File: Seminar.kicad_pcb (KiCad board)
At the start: 2 copper layers, 185.7 x 157.2 mm, 40 parts, among them J1 Screw_Terminal_01x02, J1 USB_B_Mini, SW1 SW_Push, SW2 SW_Push, U1 NUCLEO64-F446RE, U2 PCF8574AP, U3 LM2574N-5, U3 TPS61023DRLR, U4 TP4056

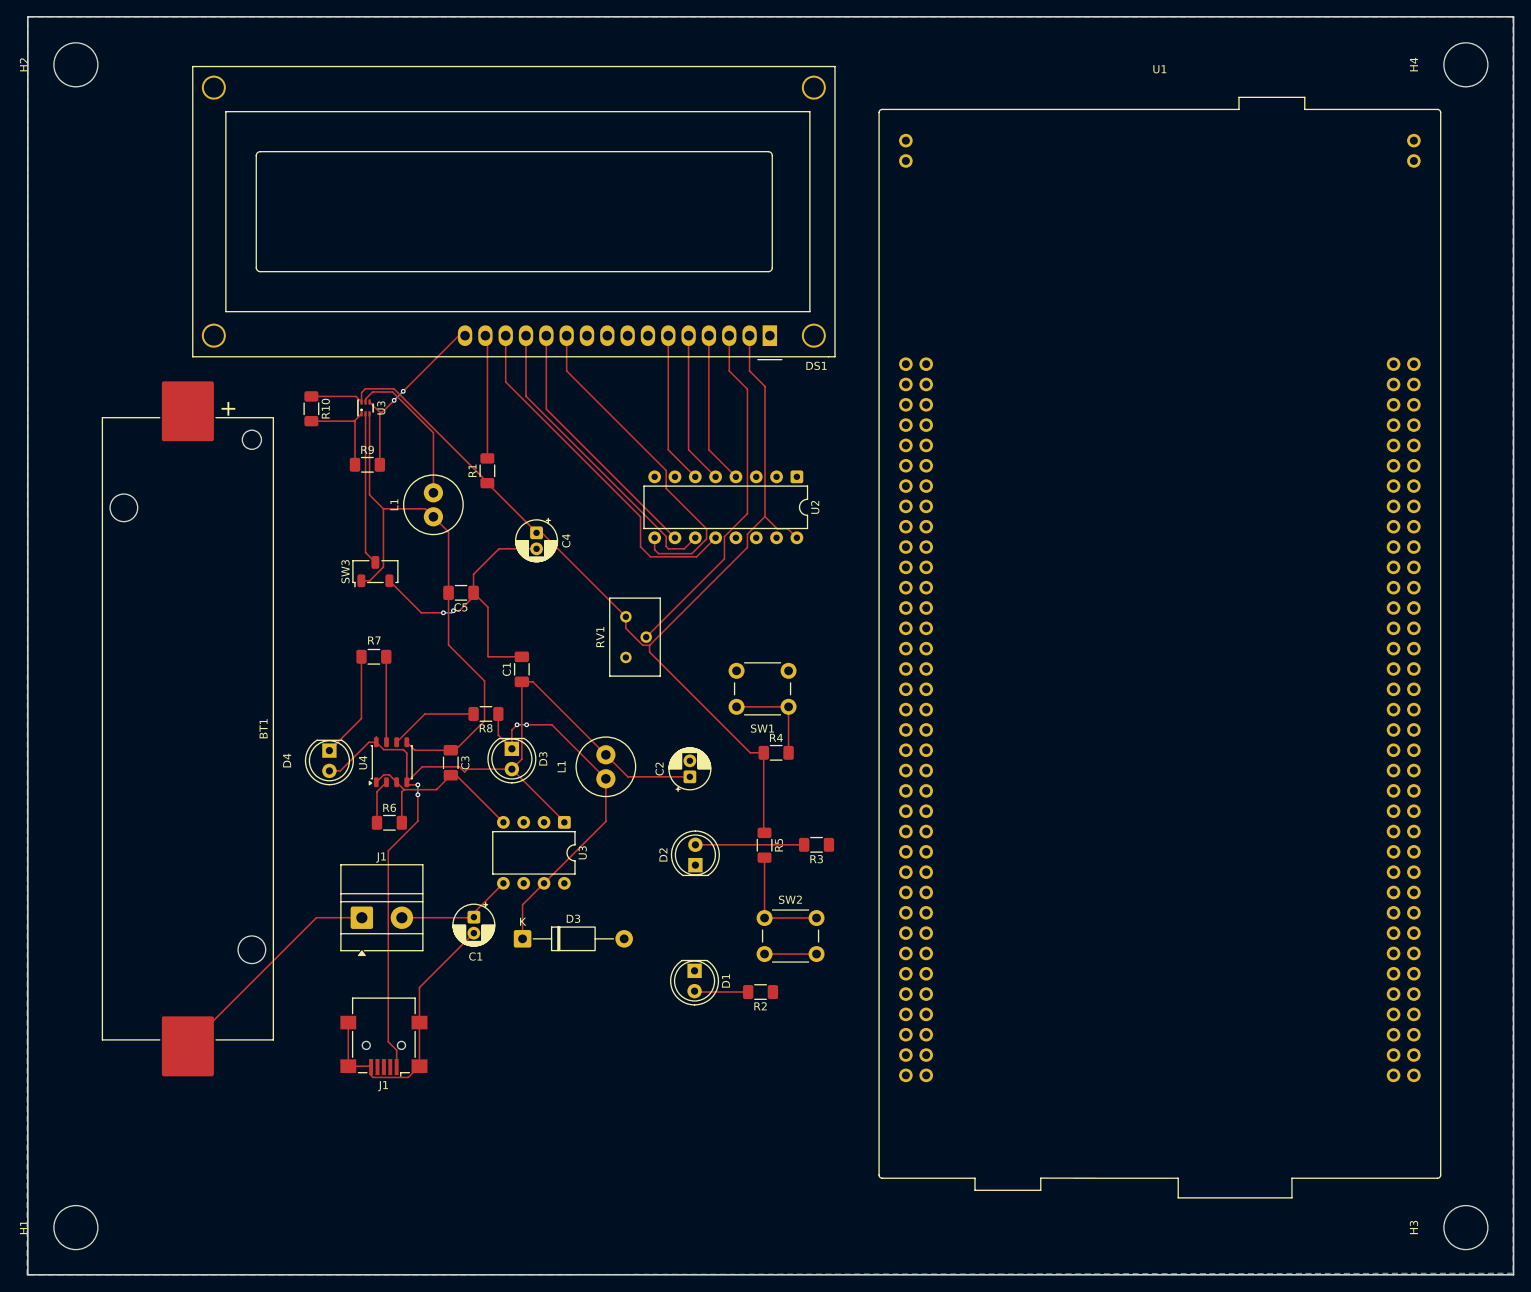
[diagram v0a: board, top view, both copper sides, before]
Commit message: Word
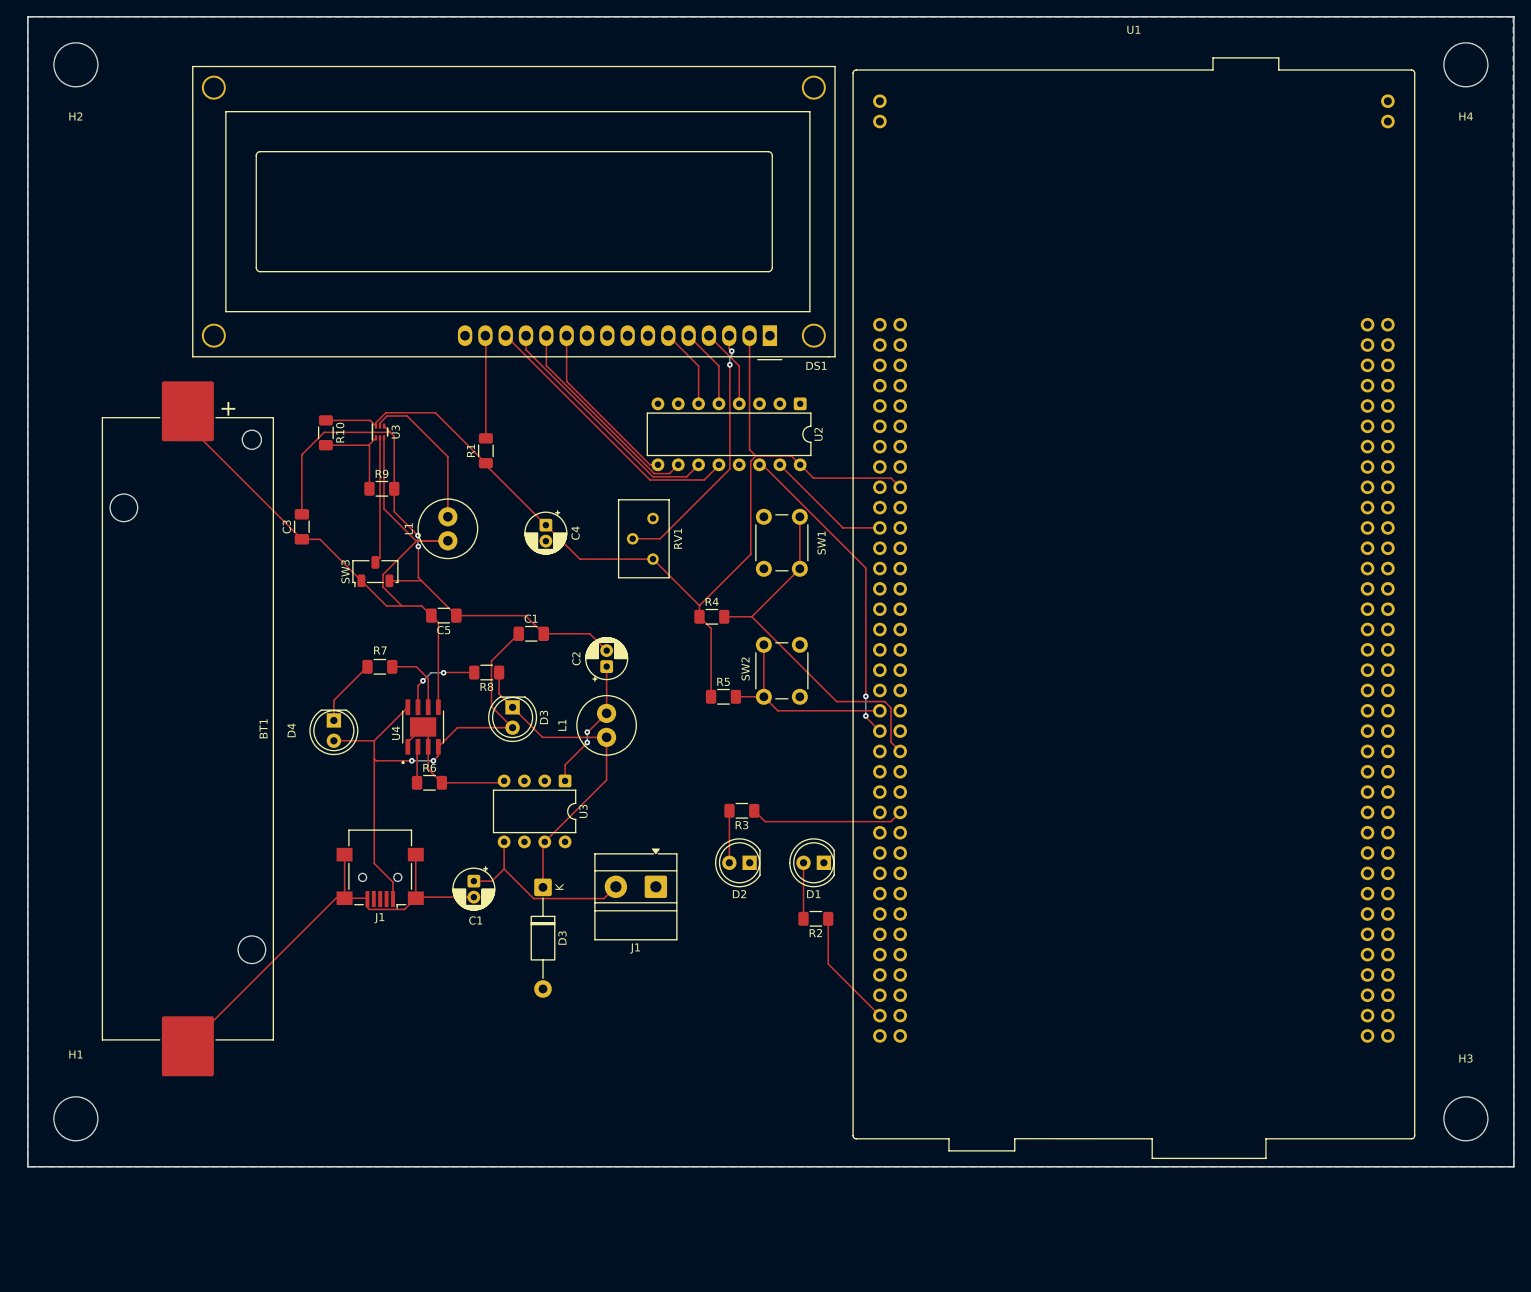
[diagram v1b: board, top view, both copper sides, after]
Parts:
- U4: footprint Package_SO:SOIC-8-1EP_3.9x4.9mm_P1.27mm_EP2.41x3.3mm_ThermalVias -> SOP127P600X175-9N:SOP127P600X175-9N
- moved J1 37.0 mm to (97.2, 126.2), turned to 180 degrees
- moved C3 34.9 mm to (53.0, 81.2), turned to 90 degrees
- moved SW2 27.7 mm to (110.8, 102.5), turned to 90 degrees
- moved SW1 23.8 mm to (115.2, 80.0), turned to -90 degrees
- moved D1 21.1 mm to (118.2, 123.2), turned to 180 degrees
- moved J1 21.0 mm to (62.8, 125.1)
- moved R5 19.3 mm to (105.7, 102.5), turned to 0 degrees
- moved R4 18.8 mm to (104.2, 92.5)
- moved C2 17.3 mm to (91.1, 98.7)
- moved H1 13.6 mm to (24.8, 155.2), turned to 180 degrees
- moved H3 13.6 mm to (198.5, 155.2), turned to 180 degrees
- moved R2 11.5 mm to (117.2, 130.2)
- moved R3 10.3 mm to (108.0, 116.8)
- moved U2 9.13 mm to (115.3, 65.9)
- moved RV1 7.97 mm to (96.9, 85.3), turned to -90 degrees
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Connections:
- R7 pad 2: Net-(U4-~{CHRG}) -> STDBY
- R8 pad 2: Net-(U4-~{STDBY}) -> CHRG
- U1 pad 21: unconnected-(U1-PB7-Pad21) -> SDA
- U1 pad 39: unconnected-(U1-PC9-Pad39) -> STOP
- U1 pad 43: SDA -> unconnected-(U1-PB9-Pad43)
- U1 pad 61: STOP -> unconnected-(U1-PA8-Pad61)
- U4 pad 6: Net-(U4-~{STDBY}) -> STDBY
- U4 pad 7: Net-(U4-~{CHRG}) -> CHRG
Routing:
- net +5V: track 77.1 -> 16.5 mm, vias 0 -> 2
- net SCL: track 0.00 -> 39.7 mm, vias 0 -> 2
- net START: track 12.0 -> 46.5 mm
- net USB 5V: track 38.4 -> 65.7 mm
- net Net-(DS1-D4): track 41.6 -> 21.4 mm
- net BLUE: track 0.00 -> 19.3 mm
- net +Vin: track 70.9 -> 88.2 mm
- net SDA: track 0.00 -> 15.8 mm
- net RED: track 0.00 -> 14.8 mm
- net 5V: track 139.6 -> 126.7 mm
- net Net-(DS1-VO): track 43.9 -> 32.7 mm, vias 0 -> 2
- net STOP: track 14.1 -> 25.2 mm
- net Net-(U4-~{STDBY}): track 11.1 -> 0.00 mm
- net Net-(U4-~{CHRG}): track 10.8 -> 0.00 mm
- net CHRG: track 0.00 -> 10.4 mm, vias 0 -> 2
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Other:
- board size 185.7 x 157.2 mm -> 185.8 x 143.8 mm
